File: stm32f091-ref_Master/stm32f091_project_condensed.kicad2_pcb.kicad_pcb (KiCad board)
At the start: 4 copper layers, 56 x 42.7 mm, 64 parts, among them J1 Conn_02x05_Odd_Even, J2 Conn_01x09_Female, J3 Conn_01x08_Female, J4 Conn_01x02_Female, SW1 SW_Push, SW2 SW_Push, U1 LD1117S33TR_SOT223, U2 LM324, U3 STM32F091RCTx, U4 LM386

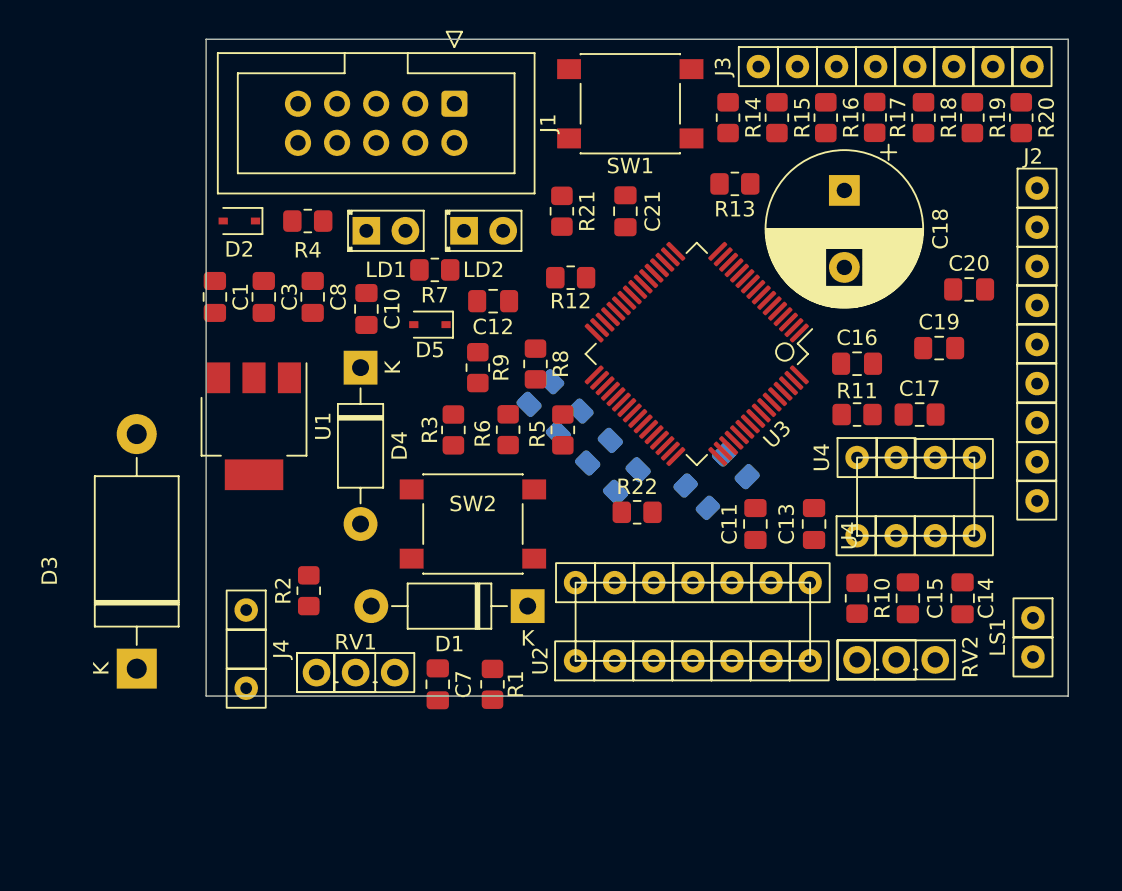
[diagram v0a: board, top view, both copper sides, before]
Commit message: new pcb design
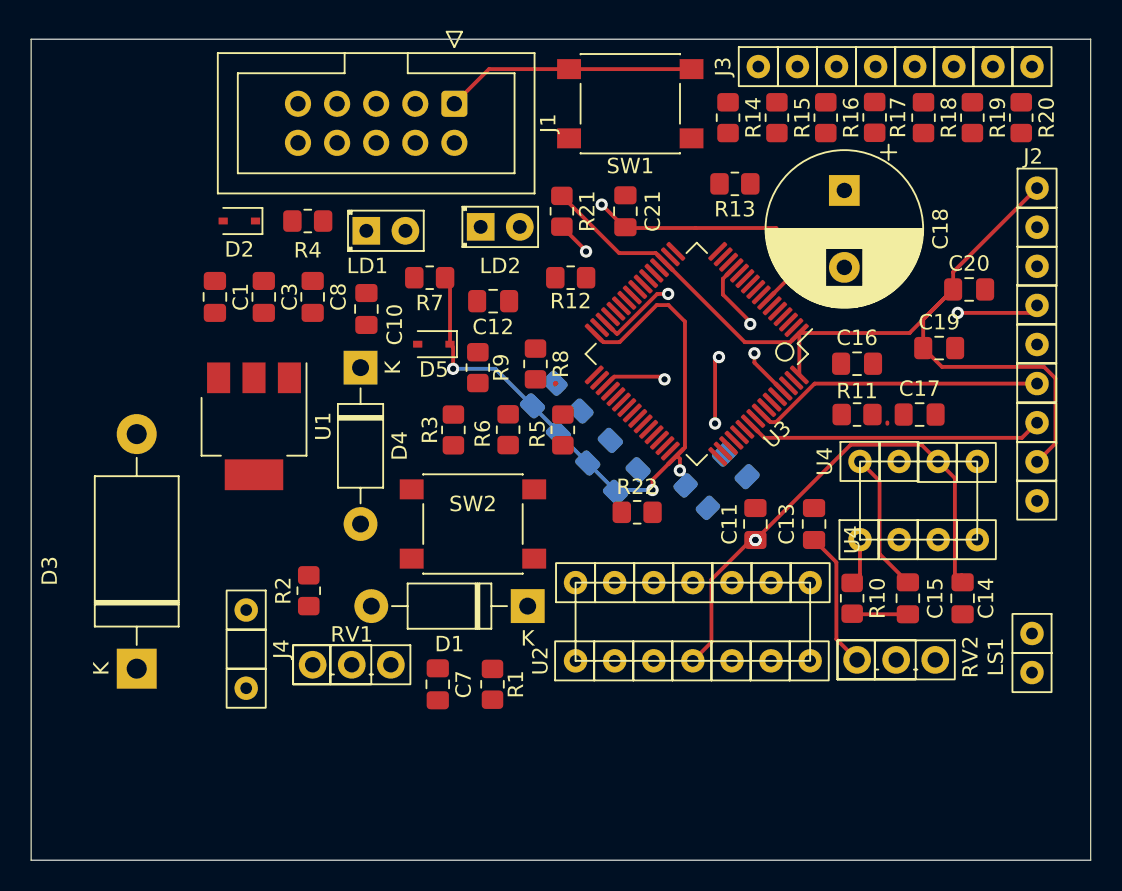
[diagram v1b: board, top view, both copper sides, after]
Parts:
- moved D5 1.30 mm to (105.2, 119.1)
- moved LD2 1.11 mm to (108.2, 111.4)
- moved LS1 1.02 mm to (144.0, 139.1)
- moved R7 0.61 mm to (104.9, 114.7)
- moved RV1 0.57 mm to (97.3, 139.9)
- moved U4 0.32 mm to (136.7, 129.2)
- moved R10 0.32 mm to (132.4, 135.6)
- moved C2 0.24 mm to (112.3, 122.3)
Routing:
- net +3V0: track 0.00 -> 133.6 mm, vias 0 -> 3
- net +5V: track 0.00 -> 88.8 mm, vias 0 -> 2
- net /NRST: track 0.00 -> 40.6 mm, vias 0 -> 2
- net PB11: track 0.00 -> 30.2 mm, vias 0 -> 2
- net PB14: track 0.00 -> 29.6 mm, vias 0 -> 1
- net PB8: track 0.00 -> 24.0 mm, vias 0 -> 1
- net /3VA: track 0.00 -> 19.8 mm, vias 0 -> 3
- net PB3: track 0.00 -> 19.4 mm
- net PB5: track 0.00 -> 19.2 mm
- net Net-(C15-Pad2): track 0.00 -> 9.14 mm
- net Net-(C13-Pad2): track 0.00 -> 8.95 mm
- net Net-(C15-Pad1): track 0.00 -> 3.64 mm
- net Net-(R10-Pad1): track 0.00 -> 3.02 mm
- net GND: track 0.00 -> 0.95 mm
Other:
- board size 56 x 42.7 mm -> 68.8 x 53.3 mm
